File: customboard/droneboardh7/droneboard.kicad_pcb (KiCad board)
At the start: 4 copper layers, 38 x 38 mm, 61 parts, among them J1 Conn_01x04, J10 Conn_01x03_Pin, J2 Conn_01x04, J3 Conn_01x08_MountingPin, J4 Conn_01x08_MountingPin, J5 USB_C_Receptacle_USB2.0_16P, J6 Conn_01x04, Q1 DMN2056U, SW1 SW_Push, SW2 SW_Push, U1 AP62300Z6, U3 STM32H743VITx, U4 ICM-42688-P, U5 SPX3819M5-L-3-3, U6 SPX3819M5-L-3-3, Y2 CSTNE20M0V53Z000R0

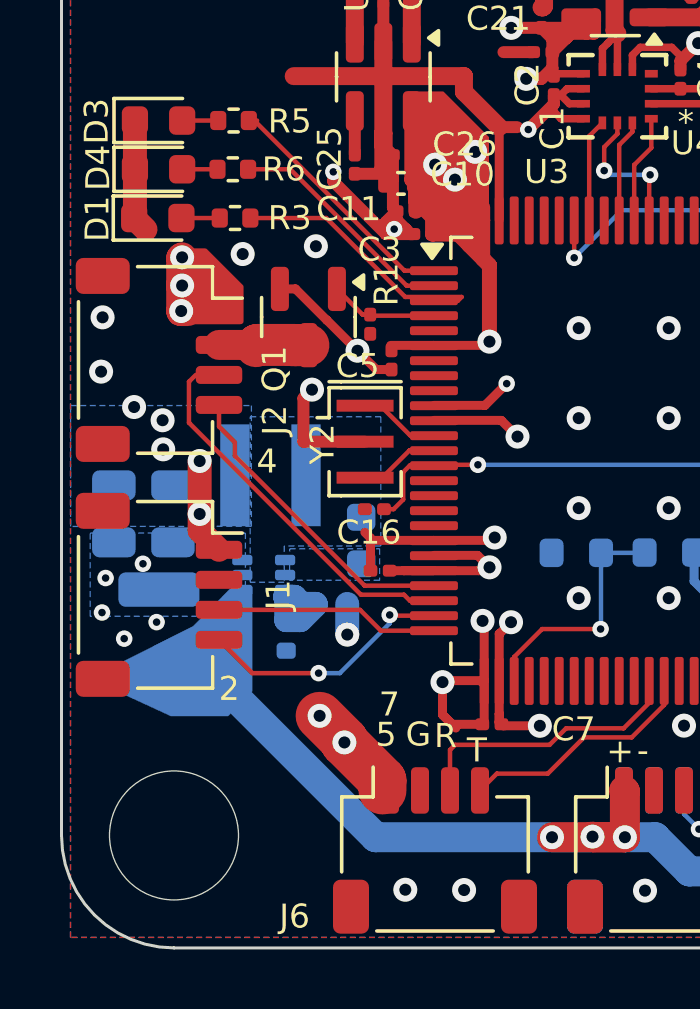
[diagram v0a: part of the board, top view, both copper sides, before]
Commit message: stuff
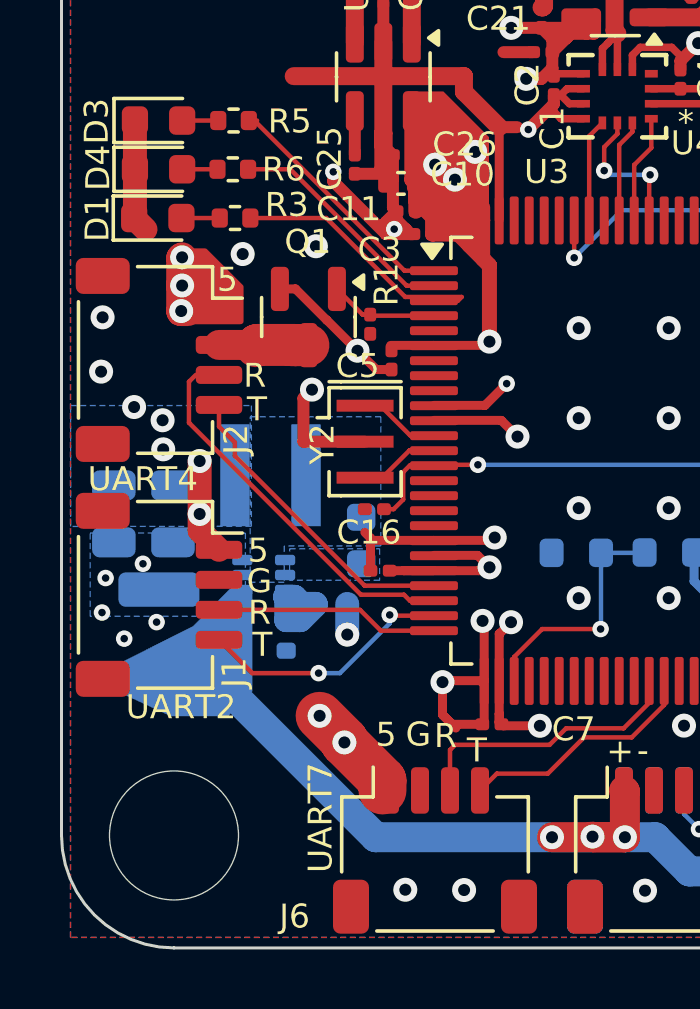
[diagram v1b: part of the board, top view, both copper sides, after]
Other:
- board text added: "UART2"
- board text added: "UART4"
- board text added: "UART7"
- board text removed: "2"
- board text removed: "4"
- board text removed: "7"
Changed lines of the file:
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@@
 			)
 		)
+		(model "${KIPRJMOD}/components/3dmodels/KMR221GLFS--3DModel-STEP-56544.STEP"
+			(offset
+				(xyz 0 0 1.5)
+			)
+			(scale
+				(xyz 1 1 1)
+			)
+			(rotate
+				(xyz -90 -0 -0)
+			)
+		)
 	)
 	(footprint "Capacitor_SMD:C_0201_0603Metric"
@@
 		(tags "connector JST SH horizontal")
 		(property "Reference" "J2"
-			(at 2.01 -3.86 90)
+			(at 2.65 -2.57 90)
 			(layer "F.SilkS")
 			(effects
@@
 			)
 		)
+		(model "${KIPRJMOD}/components/3dmodels/SM04B-SRSS-TB_LF__SN_.stp"
+			(offset
+				(xyz 0 1.25 -0.3)
+			)
+			(scale
+				(xyz 1 1 1)
+			)
+			(rotate
+				(xyz -90 -0 -0)
+			)
+		)
 	)
 	(footprint "Connector_PinHeader_2.54mm:PinHeader_1x03_P2.54mm_Vertical"
@@
 			)
 		)
+		(model "${KIPRJMOD}/components/3dmodels/USB4110GFA--3DModel-STEP-269445.STEP"
+			(offset
+				(xyz 0 2.5 0)
+			)
+			(scale
+				(xyz 1 1 1)
+			)
+			(rotate
+				(xyz -90 -0 -0)
+			)
+		)
 	)
 	(footprint "Capacitor_SMD:C_0201_0603Metric"
@@
 		(tags "resistor")
 		(property "Reference" "R3"
-			(at -1.825 0 0)
+			(at -1.725 0.44 0)
 			(layer "F.SilkS")
 			(effects
@@
 		(tags "SOT TO_SOT_SMD")
 		(property "Reference" "Q1"
-			(at 1.73 1.13 90)
+			(at -2.51 0.02 180)
 			(layer "F.SilkS")
 			(effects
@@
 		(tags "connector JST SH horizontal")
 		(property "Reference" "J1"
-			(at 0 -3.98 90)
+			(at 2.59 -2.51 90)
 			(layer "F.SilkS")
 			(effects
@@
 			)
 		)
+		(model "${KIPRJMOD}/components/3dmodels/SM04B-SRSS-TB_LF__SN_.stp"
+			(offset
+				(xyz 0 1.25 -0.3)
+			)
+			(scale
+				(xyz 1 1 1)
+			)
+			(rotate
+				(xyz -90 -0 -0)
+			)
+		)
 	)
 	(footprint "Crystal:Resonator_SMD_Murata_CSTxExxV-3Pin_3.0x1.1mm"
@@
 			)
 		)
+		(model "${KIPRJMOD}/components/3dmodels/KMR221GLFS--3DModel-STEP-56544.STEP"
+			(offset
+				(xyz 0 0 1.4)
+			)
+			(scale
+				(xyz 1 1 1)
+			)
+			(rotate
+				(xyz -90 -0 -0)
+			)
+		)
 	)
 	(footprint "Resistor_SMD:R_0402_1005Metric"
@@
 			)
 		)
+		(model "${KIPRJMOD}/components/3dmodels/SM04B-SRSS-TB_LF__SN_.stp"
+			(offset
+				(xyz 0 1.25 -0.3)
+			)
+			(scale
+				(xyz 1 1 1)
+			)
+			(rotate
+				(xyz -90 -0 -0)
+			)
+		)
 	)
 	(footprint "LED_SMD:LED_0603_1608Metric"
@@
 			)
 		)
+		(model "${KIPRJMOD}/components/3dmodels/SM08B-SRSS-TB (LF)(SN)--3DModel-STEP-269445.STEP"
+			(offset
+				(xyz 0 -2.5 1.5)
+			)
+			(scale
+				(xyz 1 1 1)
+			)
+			(rotate
+				(xyz -90 -0 -0)
+			)
+		)
 	)
 	(footprint "Package_TO_SOT_SMD:SOT-563"
@@
 			)
 		)
+		(model "${KIPRJMOD}/components/3dmodels/SM08B-SRSS-TB (LF)(SN)--3DModel-STEP-269445.STEP"
+			(offset
+				(xyz 0 -2.5 1.5)
+			)
+			(scale
+				(xyz 1 1 1)
+			)
+			(rotate
+				(xyz -90 -0 -0)
+			)
+		)
 	)
 	(footprint "Resistor_SMD:R_0402_1005Metric"
@@
 		(layer "Edge.Cuts")
 	)
+	(gr_text "5"
+		(at 55.18 98.19 0)
+		(layer "F.SilkS")
+		(effects
+			(font
+				(size 0.8 0.8)
+				(thickness 0.15)
+			)
+			(justify left bottom)
+		)
+	)
+	(gr_text "G"
+		(at 56.17 108.24 0)
+		(layer "F.SilkS")
+		(effects
+			(font
+				(size 0.8 0.8)
+				(thickness 0.15)
+			)
+			(justify left bottom)
+		)
+	)
 	(gr_text "R"
 		(at 87.6 113.02 90)
@@
 		)
 	)
+	(gr_text "R"
+		(at 56.22 109.29 0)
+		(layer "F.SilkS")
+		(effects
+			(font
+				(size 0.8 0.8)
+				(thickness 0.15)
+			)
+			(justify left bottom)
+		)
+	)
+	(gr_text "T"
+		(at 56.36 110.36 0)
+		(layer "F.SilkS")
+		(effects
+			(font
+				(size 0.8 0.8)
+				(thickness 0.15)
+			)
+			(justify left bottom)
+		)
+	)
 	(gr_text "+"
 		(at 68.16 113.91 0)
@@
 		)
 	)
-	(gr_text "2"
-		(at 55.24 111.83 0)
+	(gr_text "UART2"
+		(at 52.14 112.44 0)
+		(layer "F.SilkS")
+		(effects
+			(font
+				(size 0.8 0.8)
+				(thickness 0.15)
+			)
+			(justify left bottom)
+		)
+	)
+	(gr_text "R"
+		(at 56.06 101.39 0)
 		(layer "F.SilkS")
 		(effects
@@
 		)
 	)
-	(gr_text "7"
-		(at 60.58 112.35 0)
+	(gr_text "UART7"
+		(at 59.1 117.5 90)
+		(layer "F.SilkS")
+		(effects
+			(font
+				(size 0.8 0.8)
+				(thickness 0.15)
+			)
+			(justify left bottom)
+		)
+	)
+	(gr_text "5"
+		(at 56.21 107.22 0)
 		(layer "F.SilkS")
 		(effects
@@
 		)
 	)
-	(gr_text "4"
-		(at 56.5 104.25 0)
+	(gr_text "UART4"
+		(at 50.87 104.84 0)
 		(layer "F.SilkS")
 		(effects
@@
 		(layer "F.SilkS")
 		(effects
+			(font
+				(size 0.8 0.8)
+				(thickness 0.15)
+			)
+			(justify left bottom)
+		)
+	)
+	(gr_text "T"
+		(at 56.18 102.51 0)
+		(layer "F.SilkS")
+		(effects
